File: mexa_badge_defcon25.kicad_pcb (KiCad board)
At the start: 2 copper layers, 148.1 x 115.1 mm, 60 parts, among them P2 LiPo, P3 CONN_01X10, P4 CONN_01X10, P5 USB Serial, P6 OLED_I2C, Q1 Q_PNP_BCE, SW1 SW_RESET, SW2 SW_BOOT, SW3 SW_PUSH, SW4 SW_PUSH, U1 SPX1117, U2 MCP73831, U3 ESP-12E

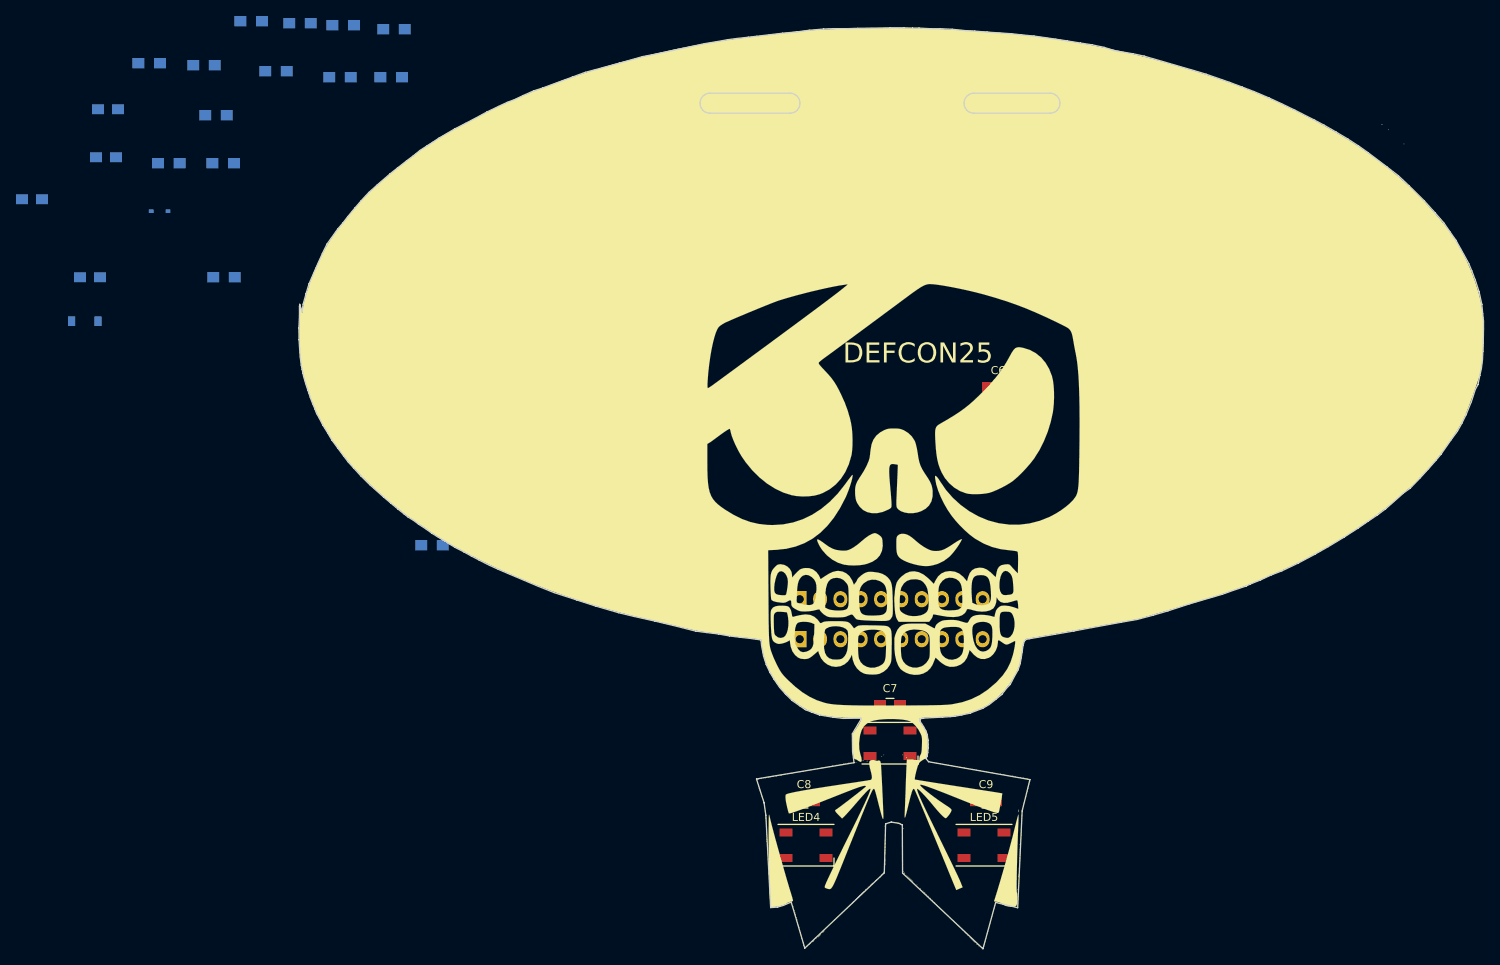
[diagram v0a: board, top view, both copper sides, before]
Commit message: Pre acomodo
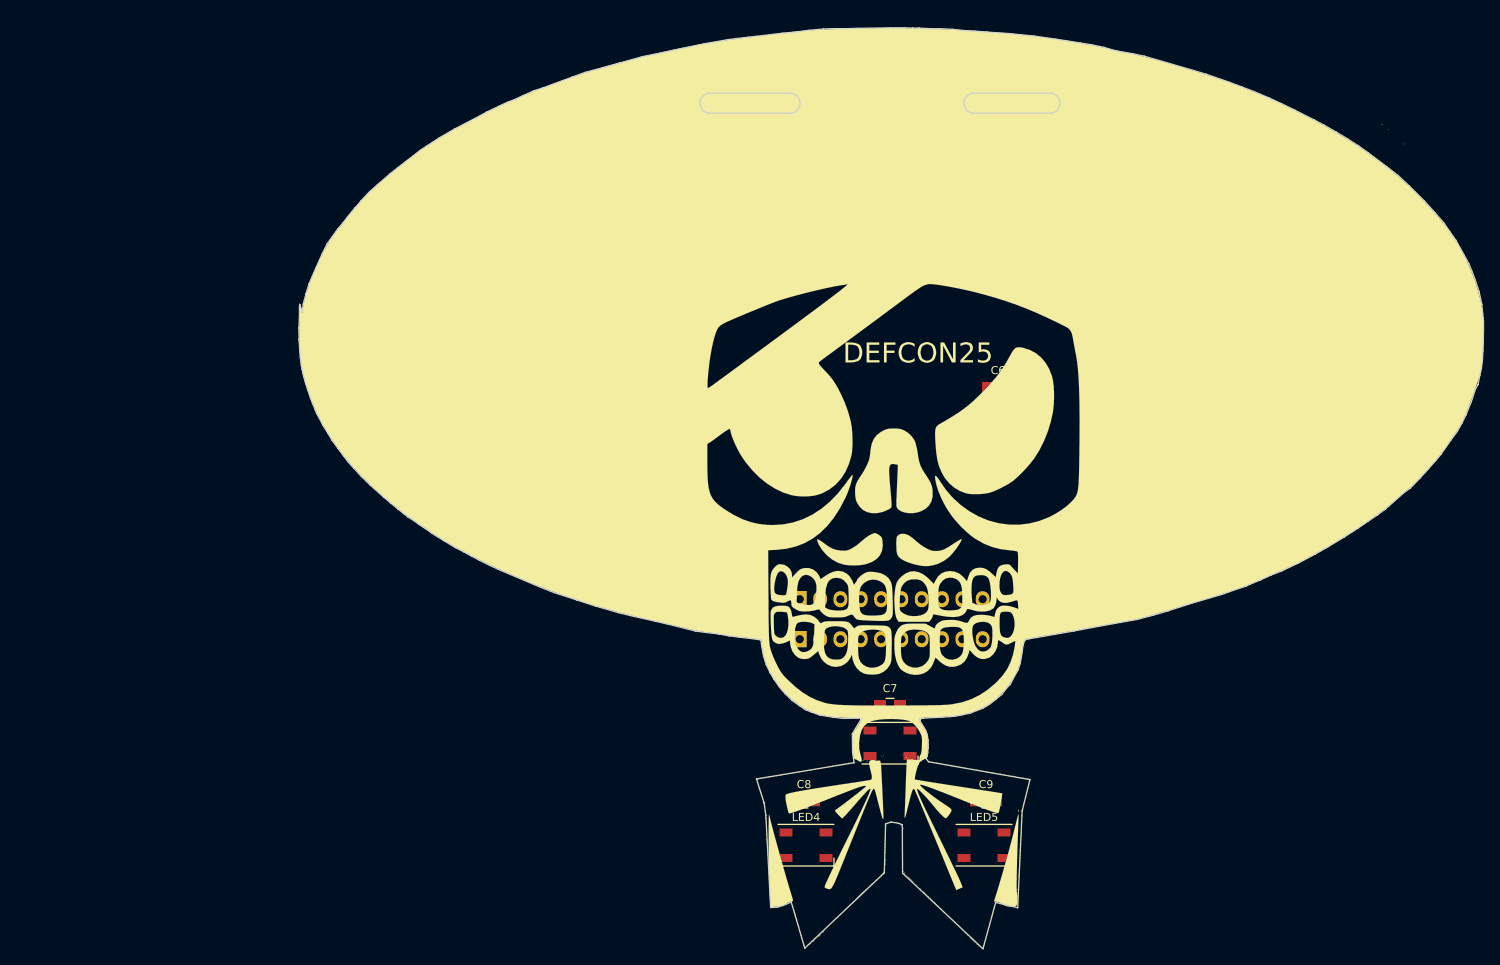
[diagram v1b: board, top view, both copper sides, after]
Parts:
- moved C1 146.0 mm to (195.0, 57.2)
- moved R3 136.6 mm to (186.0, 72.0)
- moved D3 133.2 mm to (186.0, 82.0), turned to 180 degrees
- moved R1 132.4 mm to (189.2, 57.2)
- moved R8 124.3 mm to (187.5, 76.2)
- moved R7 99.1 mm to (162.2, 36.0)
- moved R9 97.8 mm to (164.7, 41.2)
- moved R10 92.2 mm to (164.2, 46.5)
- moved R11 88.6 mm to (164.8, 51.8)
- moved R6 70.9 mm to (131.8, 45.0)
- moved R5 60.1 mm to (124.2, 45.0)
- moved D2 59.3 mm to (104.2, 80.8), turned to 90 degrees
- moved R15 55.0 mm to (108.0, 75.2)
- moved C4 51.9 mm to (93.0, 85.5), turned to 90 degrees
- moved C3 49.2 mm to (88.2, 61.5)
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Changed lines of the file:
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@@
   )
   (module Capacitors_SMD:C_0805_HandSoldering (layer B.Cu)
-    (at 49.5 45.5)
+    (at 195 57.25)
     (descr "Capacitor SMD 0805, hand soldering")
     (tags "capacitor 0805")
@@
   )
   (module Capacitors_SMD:C_0805_HandSoldering (layer B.Cu)
-    (at 49.75 39.5)
+    (at 82 70.25)
     (descr "Capacitor SMD 0805, hand soldering")
     (tags "capacitor 0805")
@@
   )
   (module Capacitors_SMD:C_0805_HandSoldering (layer B.Cu)
-    (at 40.25 50.75)
+    (at 88.25 61.5)
     (descr "Capacitor SMD 0805, hand soldering")
     (tags "capacitor 0805")
@@
   )
   (module Capacitors_SMD:C_0805_HandSoldering (layer B.Cu)
-    (at 47.5 60.5)
+    (at 93 85.5 90)
     (descr "Capacitor SMD 0805, hand soldering")
     (tags "capacitor 0805")
     (attr smd)
-    (fp_text reference C4 (at 0 2.1) (layer B.SilkS)
-      (effects (font (size 1 1) (thickness 0.15)) (justify mirror))
-    )
-    (fp_text value 10uF (at 0 -2.1) (layer B.Fab)
+    (fp_text reference C4 (at 0 2.1 90) (layer B.SilkS)
+      (effects (font (size 1 1) (thickness 0.15)) (justify mirror))
+    )
+    (fp_text value 10uF (at 0 -2.1 90) (layer B.Fab)
       (effects (font (size 1 1) (thickness 0.15)) (justify mirror))
     )
@@
     (fp_line (start 0.5 0.85) (end -0.5 0.85) (layer B.SilkS) (width 0.15))
     (fp_line (start -0.5 -0.85) (end 0.5 -0.85) (layer B.SilkS) (width 0.15))
-    (pad 1 smd rect (at -1.25 0) (size 1.5 1.25) (layers B.Cu B.Paste B.Mask)
+    (pad 1 smd rect (at -1.25 0 90) (size 1.5 1.25) (layers B.Cu B.Paste B.Mask)
       (net 7 +BATT))
-    (pad 2 smd rect (at 1.25 0) (size 1.5 1.25) (layers B.Cu B.Paste B.Mask)
+    (pad 2 smd rect (at 1.25 0 90) (size 1.5 1.25) (layers B.Cu B.Paste B.Mask)
       (net 1 GND))
     (model Capacitors_SMD.3dshapes/C_0805_HandSoldering.wrl
@@
   )
   (module Diodes_SMD:SOD-123 (layer B.Cu)
-    (at 46.85 66)
+    (at 104.25 80.75 90)
     (descr SOD-123)
     (tags SOD-123)
     (attr smd)
-    (fp_text reference D2 (at 0 2) (layer B.SilkS)
-      (effects (font (size 1 1) (thickness 0.15)) (justify mirror))
-    )
-    (fp_text value MBR120 (at 0 -2.1) (layer B.Fab)
+    (fp_text reference D2 (at 0 2 90) (layer B.SilkS)
+      (effects (font (size 1 1) (thickness 0.15)) (justify mirror))
+    )
+    (fp_text value MBR120 (at 0 -2.1 90) (layer B.Fab)
       (effects (font (size 1 1) (thickness 0.15)) (justify mirror))
     )
@@
     (fp_line (start -2.25 -1) (end 1.65 -1) (layer B.SilkS) (width 0.12))
     (fp_line (start -2.25 1) (end 1.65 1) (layer B.SilkS) (width 0.12))
-    (pad 1 smd rect (at -1.65 0) (size 0.9 1.2) (layers B.Cu B.Paste B.Mask)
+    (pad 1 smd rect (at -1.65 0 90) (size 0.9 1.2) (layers B.Cu B.Paste B.Mask)
       (net 5 VCC))
-    (pad 2 smd rect (at 1.65 0) (size 0.9 1.2) (layers B.Cu B.Paste B.Mask)
+    (pad 2 smd rect (at 1.65 0 90) (size 0.9 1.2) (layers B.Cu B.Paste B.Mask)
       (net 7 +BATT))
     (model ${KISYS3DMOD}/Diodes_SMD.3dshapes/SOD-123.wrl
@@
   )
   (module Diodes_SMD:SOD-323 (layer B.Cu)
-    (at 56.2 52.25)
+    (at 186 82 180)
     (descr SOD-323)
     (tags SOD-323)
     (attr smd)
-    (fp_text reference D3 (at 0 1.85) (layer B.SilkS)
-      (effects (font (size 1 1) (thickness 0.15)) (justify mirror))
-    )
-    (fp_text value 1N4148 (at 0.1 -1.9) (layer B.Fab)
+    (fp_text reference D3 (at 0 1.85 180) (layer B.SilkS)
+      (effects (font (size 1 1) (thickness 0.15)) (justify mirror))
+    )
+    (fp_text value 1N4148 (at 0.1 -1.9 180) (layer B.Fab)
       (effects (font (size 1 1) (thickness 0.15)) (justify mirror))
     )
@@
     (fp_line (start -1.5 -0.85) (end 1.05 -0.85) (layer B.SilkS) (width 0.12))
     (fp_line (start -1.5 0.85) (end 1.05 0.85) (layer B.SilkS) (width 0.12))
-    (pad 1 smd rect (at -1.05 0) (size 0.6 0.45) (layers B.Cu B.Paste B.Mask)
+    (pad 1 smd rect (at -1.05 0 180) (size 0.6 0.45) (layers B.Cu B.Paste B.Mask)
       (net 9 "Net-(D3-Pad1)"))
-    (pad 2 smd rect (at 1.05 0) (size 0.6 0.45) (layers B.Cu B.Paste B.Mask)
+    (pad 2 smd rect (at 1.05 0 180) (size 0.6 0.45) (layers B.Cu B.Paste B.Mask)
       (net 10 /GPIO0))
     (model Diodes_SMD.3dshapes/SOD-323.wrl
@@
   )
   (module Socket_Strips:Socket_Strip_Straight_1x02 (layer B.Cu)
-    (at 89.25 85.25)
+    (at 84.46 84.75)
     (descr "Through hole socket strip")
     (tags "socket strip")
@@
   )
   (module Resistors_SMD:R_0805_HandSoldering (layer B.Cu)
-    (at 57.35 46.25)
+    (at 189.25 57.25)
     (descr "Resistor SMD 0805, hand soldering")
     (tags "resistor 0805")
@@
   )
   (module Resistors_SMD:R_0805_HandSoldering (layer B.Cu)
-    (at 90.25 94)
+    (at 90.5 80.75)
     (descr "Resistor SMD 0805, hand soldering")
     (tags "resistor 0805")
@@
   )
   (module Resistors_SMD:R_0805_HandSoldering (layer B.Cu)
-    (at 54.9 33.75)
+    (at 186 72)
     (descr "Resistor SMD 0805, hand soldering")
     (tags "resistor 0805")
@@
   )
   (module Resistors_SMD:R_0805_HandSoldering (layer B.Cu)
-    (at 99 93.75)
+    (at 97.75 90.75)
     (descr "Resistor SMD 0805, hand soldering")
     (tags "resistor 0805")
@@
   )
   (module Resistors_SMD:R_0805_HandSoldering (layer B.Cu)
-    (at 64.15 46.25)
+    (at 124.25 45)
     (descr "Resistor SMD 0805, hand soldering")
     (tags "resistor 0805")
@@
   )
   (module Resistors_SMD:R_0805_HandSoldering (layer B.Cu)
-    (at 61.75 34)
+    (at 131.75 45)
     (descr "Resistor SMD 0805, hand soldering")
     (tags "resistor 0805")
@@
   )
   (module Resistors_SMD:R_0805_HandSoldering (layer B.Cu)
-    (at 63.25 40.25)
+    (at 162.25 36)
     (descr "Resistor SMD 0805, hand soldering")
     (tags "resistor 0805")
@@
   )
   (module Resistors_SMD:R_0805_HandSoldering (layer B.Cu)
-    (at 64.25 60.5)
+    (at 187.5 76.25)
     (descr "Resistor SMD 0805, hand soldering")
     (tags "resistor 0805")
@@
   )
   (module Resistors_SMD:R_0805_HandSoldering (layer B.Cu)
-    (at 67.65 28.5)
+    (at 164.65 41.25)
     (descr "Resistor SMD 0805, hand soldering")
     (tags "resistor 0805")
@@
   )
   (module Resistors_SMD:R_0805_HandSoldering (layer B.Cu)
-    (at 73.75 28.75)
+    (at 164.25 46.5)
     (descr "Resistor SMD 0805, hand soldering")
     (tags "resistor 0805")
@@
   )
   (module Resistors_SMD:R_0805_HandSoldering (layer B.Cu)
-    (at 79.15 29)
+    (at 164.75 51.75)
     (descr "Resistor SMD 0805, hand soldering")
     (tags "resistor 0805")
@@
   )
   (module Resistors_SMD:R_0805_HandSoldering (layer B.Cu)
-    (at 85.5 29.5)
+    (at 126 54.5)
     (descr "Resistor SMD 0805, hand soldering")
     (tags "resistor 0805")
@@
   )
   (module Resistors_SMD:R_0805_HandSoldering (layer B.Cu)
-    (at 85.15 35.5)
+    (at 125.65 60.5)
     (descr "Resistor SMD 0805, hand soldering")
     (tags "resistor 0805")
@@
   )
   (module Resistors_SMD:R_0805_HandSoldering (layer B.Cu)
-    (at 78.75 35.5)
+    (at 108 68.75)
     (descr "Resistor SMD 0805, hand soldering")
     (tags "resistor 0805")
@@
   )
   (module Resistors_SMD:R_0805_HandSoldering (layer B.Cu)
-    (at 70.75 34.75)
+    (at 108 75.25)
     (descr "Resistor SMD 0805, hand soldering")
     (tags "resistor 0805")
@@
   )
   (module TO_SOT_Packages_SMD:SOT-223 (layer B.Cu)
-    (at 109.75 87.75)
+    (at 90.5 69.25)
     (descr "module CMS SOT223 4 pins")
     (tags "CMS SOT")
@@
   )
   (module TO_SOT_Packages_SMD:SOT-23-5 (layer B.Cu)
-    (at 97.75 86.5)
+    (at 98 85)
     (descr "5-pin SOT23 package")
     (tags SOT-23-5)
